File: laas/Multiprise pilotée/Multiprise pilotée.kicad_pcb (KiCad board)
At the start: 2 copper layers, 38 parts, among them J1 Conn_01x03, J2 Conn_01x02, J3 Conn_01x02, J4 Conn_01x02, J5 Conn_01x02, J6 Conn_01x03, J7 Conn_02x06_Odd_Even, K1 Omron Relay, K2 Omron Relay, K3 Omron Relay, K4 Omron Relay, Q1 DMN2020LSN-7, Q2 DMN2020LSN-7, Q3 SSM3J355R,LF, Q4 DMN2020LSN-7, Q5 DMN2020LSN-7, Q6 SSM3J355R,LF, Q7 DMN2020LSN-7, Q8 DMN2020LSN-7, U1 MAX4820xUP, U2 74HC595, U3 TPS75933KC, U4 TC4469, U5 TC4469, U6 TDA7391PD, U7 74AHC1G08, U8 MOUDLE-SEEEDUINO-XIAO

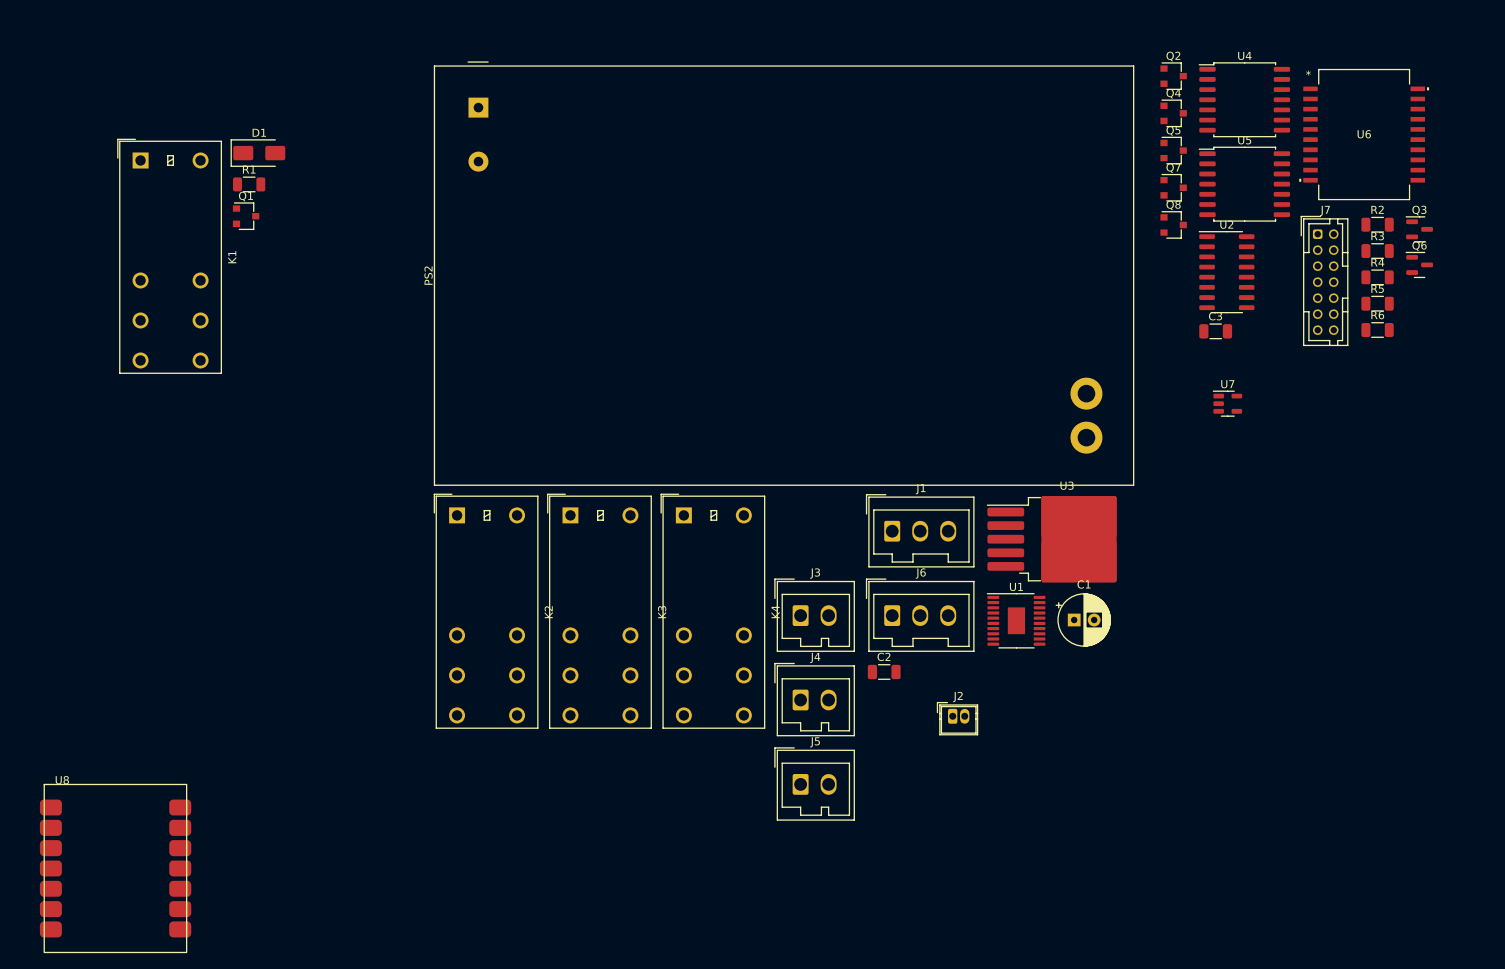
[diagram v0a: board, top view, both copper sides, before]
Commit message: Commit de propreté
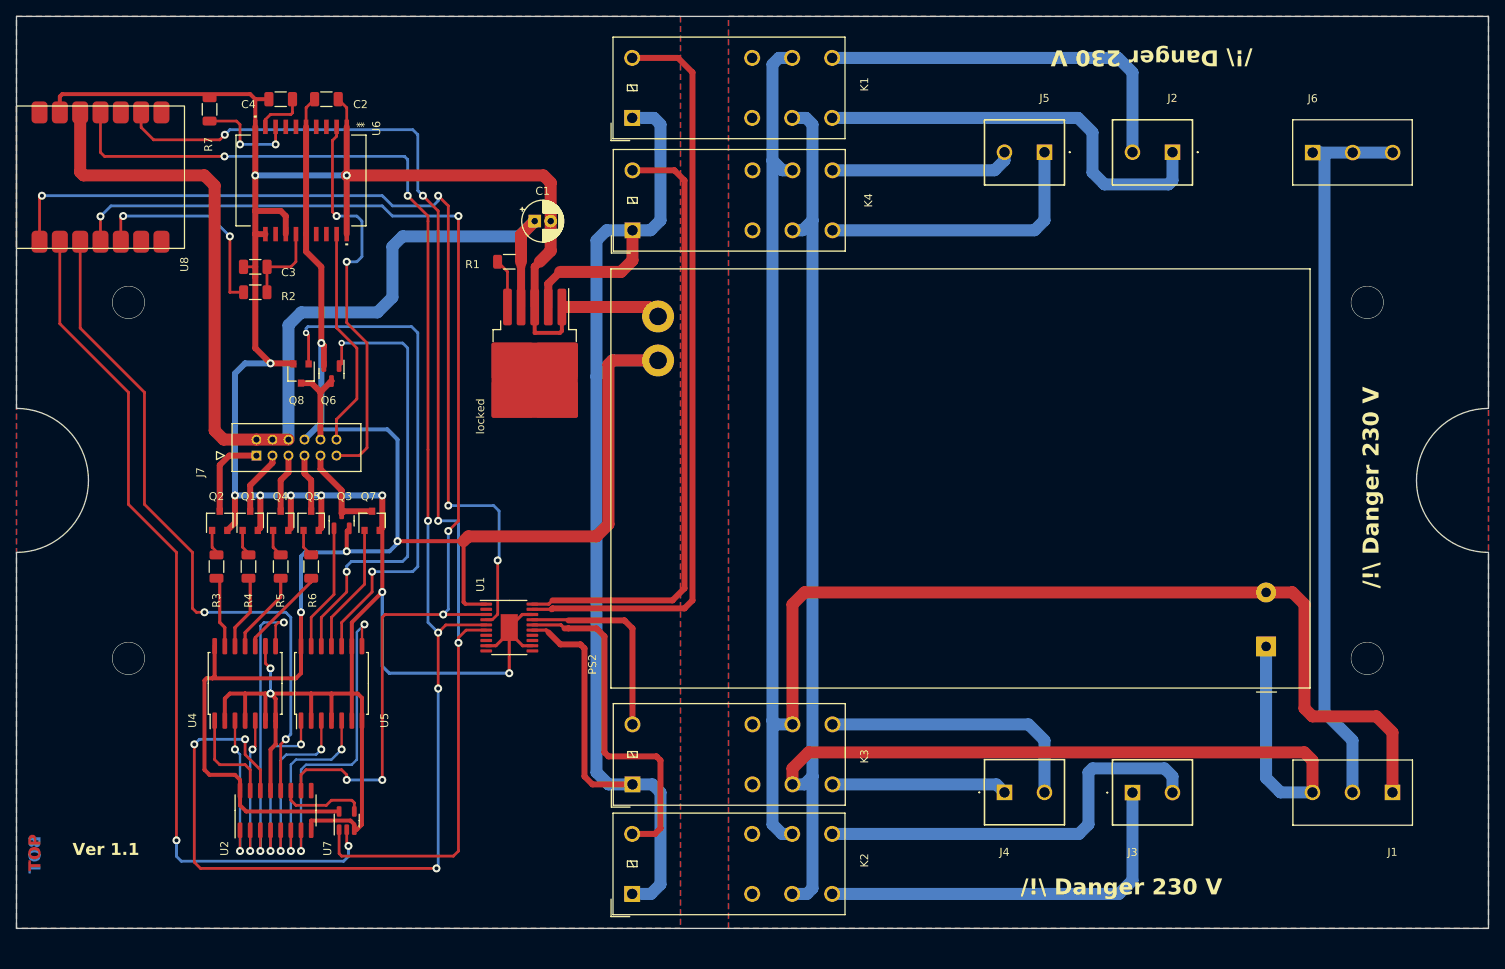
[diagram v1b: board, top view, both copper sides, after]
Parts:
- removed D1: D_Schottky, Diode_SMD:D_SMA
- added C4: 33µF, Capacitor_SMD:C_1206_3216Metric, F.Cu at (90.0, 47.4)
- added R7: 56K, Resistor_SMD:R_1206_3216Metric, F.Cu at (81.1, 48.6)
- C1: footprint Capacitor_THT:CP_Radial_D6.3mm_P2.50mm -> Capacitor_THT:CP_Radial_D5.0mm_P2.00mm
- J1, J6: footprint Connector_Wago:Wago_734-133_1x03_P3.50mm_Vertical -> Borniers:5442183
- J2: footprint Connector_Wuerth:Wuerth_WR-WTB_64800211622_1x02_P1.50mm_Vertical -> Borniers:5442170
- J3, J4, J5: footprint Connector_Wago:Wago_734-132_1x02_P3.50mm_Vertical -> Borniers:5442170
- J7: footprint Connector_JAE:JAE_LY20-14P-DT1_2x07_P2.00mm_Vertical -> Borniers:M80-85312YY
- moved R3 150.4 mm to (82.0, 105.8), turned to 90 degrees
- moved R4 145.7 mm to (86.0, 105.8), turned to 90 degrees
- moved U4 144.7 mm to (85.6, 120.4), turned to 90 degrees
- moved R5 141.0 mm to (90.0, 105.8), turned to 90 degrees
- moved R2 140.5 mm to (86.8, 71.5)
- moved Q3 139.6 mm to (97.6, 100.1), turned to 90 degrees
- moved Q6 136.7 mm to (96.4, 81.6), turned to -90 degrees
- moved U2 136.6 mm to (89.4, 136.2), turned to 90 degrees
- moved R6 136.5 mm to (93.8, 105.8), turned to 90 degrees
- moved J7 135.5 mm to (87.0, 91.9), turned to 180 degrees
- moved U6 133.0 mm to (92.6, 57.5), turned to -90 degrees
- moved Q2 131.6 mm to (82.4, 100.1), turned to 90 degrees
- moved U5 130.1 mm to (96.4, 120.4), turned to 90 degrees
- moved Q4 122.7 mm to (90.0, 100.1), turned to 90 degrees
- moved U7 121.8 mm to (98.3, 137.5), turned to 90 degrees
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- renumbered U3 to locked
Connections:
- U1 pad 16: /Power supply and relays/Relay_4 -> /Power supply and relays/Relay_2
- U1 pad 19: /Power supply and relays/Relay_2 -> /Power supply and relays/Relay_1
- U1 pad 20: /Power supply and relays/Relay_1 -> /Power supply and relays/Relay_4
- U6 pad 8: unconnected-(U6-SYNC-Pad8) -> Net-(U6-SYNC)
- U6 pad 9: unconnected-(U6-MUTE-Pad9) -> Net-(U6-MUTE)
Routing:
- net +5V: track 0.00 -> 389.2 mm, vias 0 -> 4
- net GND: track 0.00 -> 374.4 mm, vias 0 -> 12
- net NEUT: track 0.00 -> 219.5 mm
- net LINE: track 0.00 -> 202.4 mm
- net /DC supplies/MOSI: track 0.00 -> 199.6 mm, vias 0 -> 8
- net /DC supplies/SCLK: track 0.00 -> 153.8 mm, vias 0 -> 4
- net /DC supplies/~{RESET_IO}: track 0.00 -> 146.3 mm, vias 0 -> 6
- net +3V3: track 0.00 -> 130.9 mm
- net /MCU/~{CS_RELAY}: track 0.00 -> 117.4 mm, vias 0 -> 4
- net /DC supplies/CS_PWR_DC: track 0.00 -> 108.4 mm, vias 0 -> 2
- net /Power supply and relays/Relay_1: track 0.00 -> 94.8 mm
- net Earth: track 0.00 -> 91.6 mm
- net /DC supplies/LATCH: track 0.00 -> 86.6 mm, vias 0 -> 2
- net /Power supply and relays/Relay_4: track 0.00 -> 77.8 mm
- net Net-(Q8-G): track 0.00 -> 65.0 mm, vias 0 -> 2
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- added copper zone on B.Cu, net GND
- added copper zone on F.Cu, net GND
- added copper zone on B.Cu, net NEUT
- added copper zone on F.Cu, net NEUT
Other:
- board outline added: 184 x 114 mm
- board text added: "/!\ Danger 230 V"
- board text added: "BOT"
- board text added: "TOP"
- board text added: "Ver 1.1"
